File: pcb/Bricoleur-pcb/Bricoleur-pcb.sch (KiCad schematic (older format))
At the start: 29 parts, among them J1 USB_B_Micro, SW2 SW_Push, U11 SW_DP3T, U2 PYNQ-Shield-Bricoleur-pcb-cac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, U5 Arducam-OV5642, U6 Arducam-OV5642, U7 EFM32GG980, U8 UART_BOOT, U9 IP4220CZ6

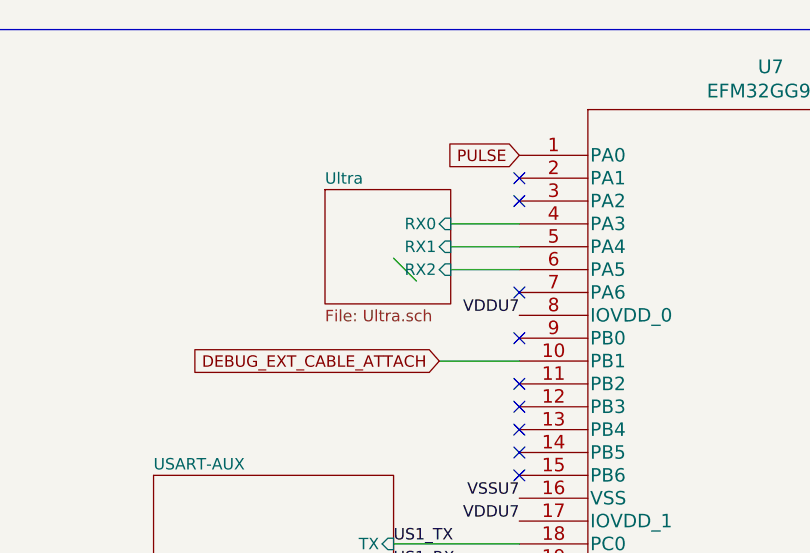
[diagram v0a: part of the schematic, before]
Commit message: PCB…
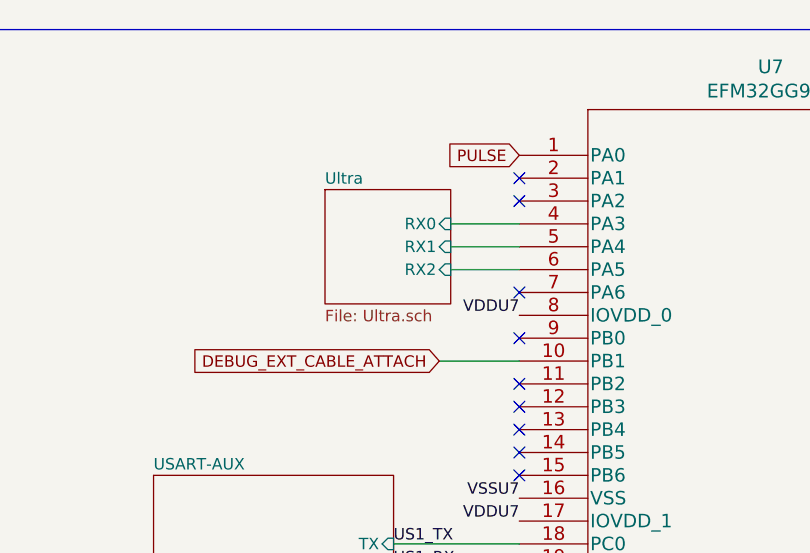
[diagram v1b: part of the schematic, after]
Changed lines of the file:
@@
 $EndComp
-Wire Wire Line
-	9300 1750 9300 2750
 Wire Wire Line
 	10700 1850 9400 1850
@@
 	-1   0    0    1
 $EndComp
-Wire Wire Line
-	9750 2750 9300 2750
-Connection ~ 9300 2750
 Text Label 11150 2550 1    50   ~ 0
 GND
 Wire Wire Line
 	11150 2750 11150 3000
-Wire Wire Line
-	11150 3000 9600 3000
-Connection ~ 9600 3000
 Wire Wire Line
 	9600 3000 9600 2050
@@
 $EndSheet
 Wire Wire Line
-	9300 2750 9300 3350
-Wire Wire Line
 	10700 2050 9600 2050
 $Sheet
@@
 F4 "TX" I R 2450 1700 50
 $EndSheet
-Entry Wire Line
-	5600 1650 5700 1750
 Entry Wire Line
 	2900 1400 3000 1500
@@
 Wire Wire Line
 	8350 1800 8750 1800
+Connection ~ 8750 1550
+Wire Bus Line
+	2900 3600 2900 4850
+Wire Bus Line
+	3000 6250 4850 6250
+Wire Bus Line
+	2900 5100 2900 6550
+Wire Bus Line
+	2900 6550 4850 6550
+Wire Bus Line
+	3000 650  3000 4750
+Wire Bus Line
+	3050 4750 3050 5650
+Wire Bus Line
+	8950 2700 8950 4200
+Wire Wire Line
+	2350 5200 2950 5200
+Wire Wire Line
+	8350 4000 9050 4000
 Wire Wire Line
 	2350 5700 2950 5700
 Wire Wire Line
-	8350 4000 9050 4000
-Wire Wire Line
-	2350 5200 2950 5200
-Wire Bus Line
-	8950 2700 8950 4200
-Wire Bus Line
-	3050 4750 3050 5650
-Wire Bus Line
-	3000 650  3000 4750
-Wire Bus Line
-	2900 6550 4850 6550
-Wire Bus Line
-	2900 5100 2900 6550
-Wire Bus Line
-	3000 6250 4850 6250
-Wire Bus Line
-	2900 3600 2900 4850
-Connection ~ 8750 1550
+	11150 3000 9600 3000
+Connection ~ 9600 3000
+Wire Wire Line
+	9300 2750 9300 3350
+Wire Wire Line
+	9300 1750 9300 2750
+Connection ~ 9300 2750
+Wire Wire Line
+	9750 2750 9300 2750
 $EndSCHEMATC
